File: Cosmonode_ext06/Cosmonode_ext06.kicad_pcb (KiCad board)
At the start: 2 copper layers, 24.1 x 33 mm, 19 parts, among them J1 CONN_01X04, J2 CONN_01X04, J3 CONN_01X08, J4 CONN_01X08, J5 GS3, J6 GS3, Q1 BSS138, Q2 BSS138, SW1 SW_Push, SW2 SW_Push, U1 XC6206P502MR

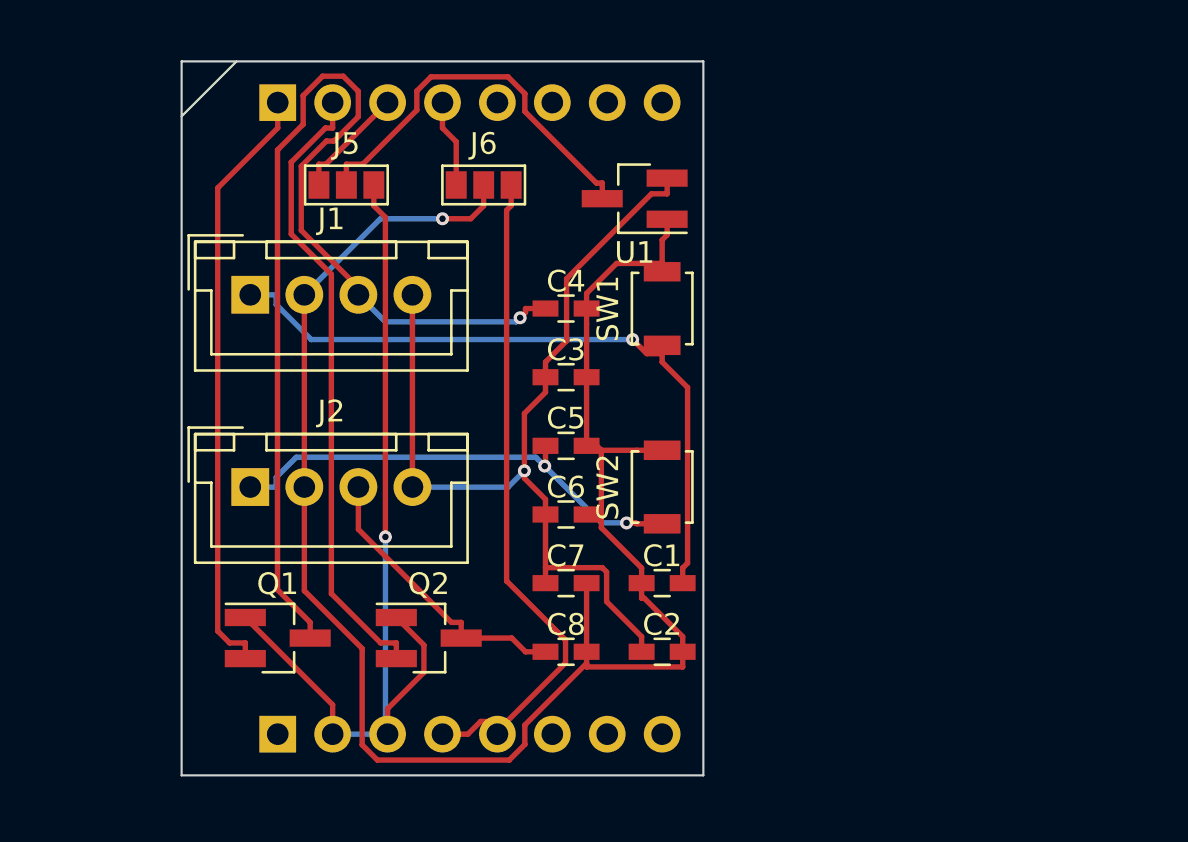
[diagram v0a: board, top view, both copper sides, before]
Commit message: big push2
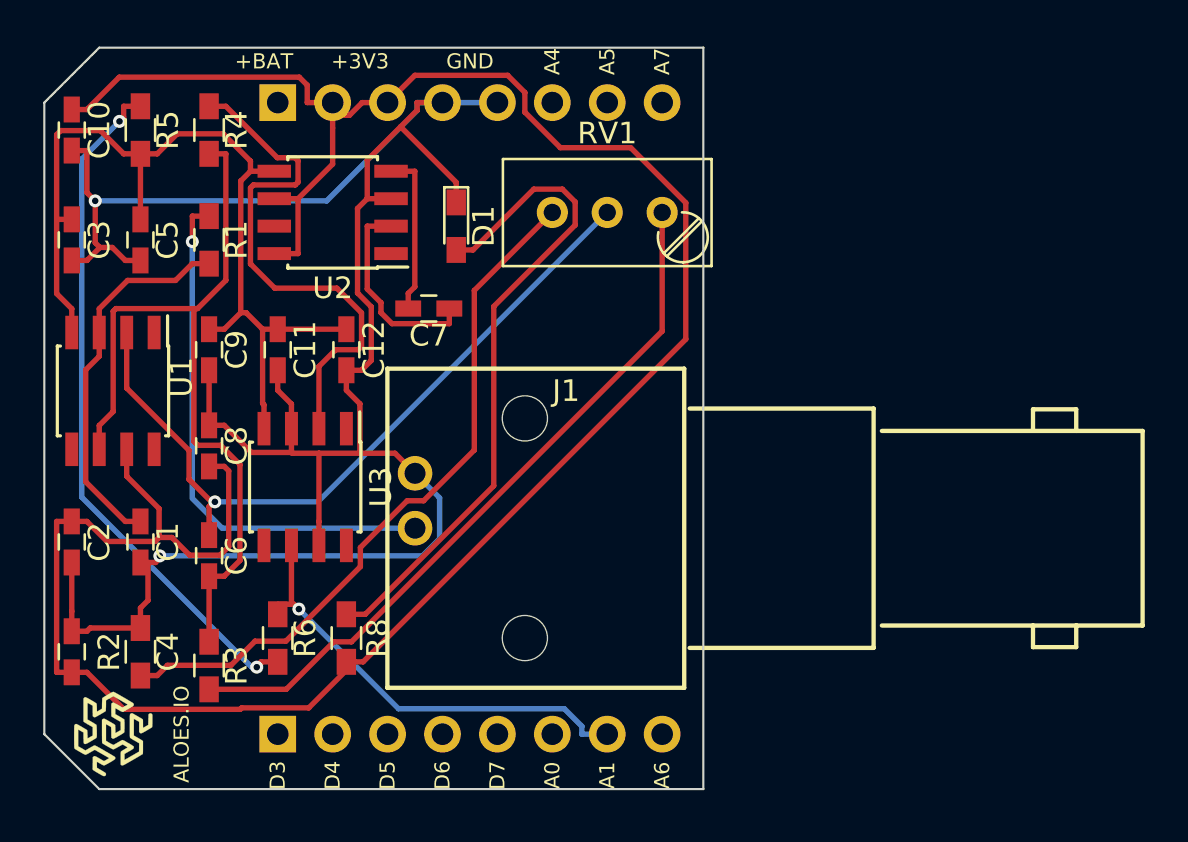
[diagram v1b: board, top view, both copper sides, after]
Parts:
- removed J5: GS3, Connectors:GS3
- removed Q1, Q2: BSS138, TO_SOT_Packages_SMD:SOT-23_Handsoldering
- removed SW1, SW2: SW_Push, Buttons_Switches_SMD:SW_SPST_B3U-1000P
- added C10: 100nF, Capacitors_SMD:C_0603_HandSoldering, F.Cu at (149.2, 92.7)
- added C11: 100nF, Capacitors_SMD:C_0603_HandSoldering, F.Cu at (158.8, 102.9)
- added C12: 100uF, Capacitors_SMD:C_0603_HandSoldering, F.Cu at (161.9, 102.9)
- added C9: 10uF, Capacitors_SMD:C_0603_HandSoldering, F.Cu at (155.6, 102.9)
- added D1: LED, LEDs:LED_0603_HandSoldering, F.Cu at (167.0, 97.2)
- added R1: 4,7M, Resistors_SMD:R_0603_HandSoldering, F.Cu at (155.6, 97.8)
- added R2: 1k, Resistors_SMD:R_0603_HandSoldering, F.Cu at (152.4, 116.8)
- added R3: 2,2k, Resistors_SMD:R_0603_HandSoldering, F.Cu at (155.6, 117.5)
- added R4: 30k, Resistors_SMD:R_0603_HandSoldering, F.Cu at (155.6, 92.7)
- added R5: 75k, Resistors_SMD:R_0603_HandSoldering, F.Cu at (152.4, 92.7)
- added R6: 30k, Resistors_SMD:R_0603_HandSoldering, F.Cu at (158.8, 116.2)
- added R8: 1k, Resistors_SMD:R_0603_HandSoldering, F.Cu at (161.9, 116.2)
- added RV1: 5k, Potentiometers:Potentiometer_Trimmer_Bourns_3296W, F.Cu at (176.5, 96.5)
- added U2: ICL7660AIBAZA, Housings_SOIC:SOIC-8_3.9x4.9mm_Pitch1.27mm, F.Cu at (161.3, 96.5)
- added U3: TL081BCD, Housings_SOIC:SOIC-8_3.9x4.9mm_Pitch1.27mm, F.Cu at (160.0, 109.2)
- C1: value 100nF -> 2,2nF
- C2: value 10uF -> 100nF
- C3, C4, C8: value 100nF -> 10uF
- C6: value 10uF -> 1uF
- C7: value 100nF -> 100uF
- J1: value CONN_01X04 -> 227161-1; footprint Connectors_JST:JST_XH_B04B-XH-A_04x2.50mm_Straight -> BNC_P7003:TE_227161-1
- J2: value CONN_01X04 -> Aloes_Logo; footprint Connectors_JST:JST_XH_B04B-XH-A_04x2.50mm_Straight -> Aloes:Aloes_mini
- J3: value CONN_01X08 -> OSHW_Logo; footprint Pin_Headers:Pin_Header_Straight_1x08_Pitch2.54mm -> Symbols:OSHW-Logo_5.7x6mm_SilkScreen
- J4: footprint Pin_Headers:Pin_Header_Straight_1x08_Pitch2.54mm -> Socket_Strips:Socket_Strip_Straight_1x08_Pitch2.54mm
- J6: value GS3 -> CONN_01X08; footprint Connectors:GS3 -> Socket_Strips:Socket_Strip_Straight_1x08_Pitch2.54mm; moved to B.Cu
- U1: value XC6206P502MR -> CA3140AMZ; footprint TO_SOT_Packages_SMD:SOT-23_Handsoldering -> Housings_SOIC:SOIC-8_3.9x4.9mm_Pitch1.27mm
- moved C4 27.8 mm to (149.2, 116.8), turned to 90 degrees
- moved C2 27.8 mm to (149.2, 111.8), turned to 90 degrees
- moved U1 25.7 mm to (151.1, 104.8), turned to 270 degrees
- moved C1 24.2 mm to (152.4, 111.8), turned to 90 degrees
- moved C3 23.7 mm to (149.2, 97.8), turned to 90 degrees
- moved C5 21.9 mm to (152.4, 97.8), turned to 270 degrees
- moved C8 19.1 mm to (155.6, 107.3), turned to 90 degrees
- moved J1 16.7 mm to (170.2, 111.1), turned to 270 degrees
- moved C6 16.6 mm to (155.6, 112.4), turned to 90 degrees
- moved C7 14.2 mm to (165.7, 101.0), turned to 180 degrees
- moved J2 13.1 mm to (151.1, 120.7), turned to 90 degrees
- moved J6 10.3 mm to (158.8, 91.4), turned to 270 degrees
- moved J3 7.24 mm to (153.0, 95.9)
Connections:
- C1 pad 1: Net-(C1-Pad1) -> GND
- C2 pad 1: +5V -> GND
- C2 pad 2: Net-(C1-Pad1) -> +3V3
- C3 pad 1: +5V -> GND
- C3 pad 2: Net-(C1-Pad1) -> -3V3
- C4 pad 1: /D3_5V -> +3V3
- C4 pad 2: Net-(C1-Pad1) -> GND
- C5 pad 1: Net-(C1-Pad1) -> -3V3
- C5 pad 2: Net-(C5-Pad2) -> GND
- C6 pad 1: +5V -> Net-(C6-Pad1)
- C6 pad 2: Net-(C1-Pad1) -> Net-(C6-Pad2)
- C7 pad 1: +5V -> Net-(C7-Pad1)
- C7 pad 2: Net-(C1-Pad1) -> Net-(C7-Pad2)
- C8 pad 1: /D4_5V -> +3V3
- C8 pad 2: Net-(C1-Pad1) -> GND
- J1 pad 1: Net-(C1-Pad2) -> GND
- J1 pad 2: Net-(C1-Pad1) -> Net-(J1-Pad2)
- J4 pad 1: /BAT+ -> /D3
- J4 pad 2: +3V3 -> /D4
- J4 pad 3: +3V3 -> /D5
- J4 pad 4: GND -> /D6
- J4 pad 5: GND -> /D7
- J4 pad 6: /A4 -> /A0
- J4 pad 7: /A5 -> /A1
- J4 pad 8: /A7 -> /A6
- J6 pad 1: /D6 -> /BAT+
- J6 pad 2: Net-(C1-Pad1) -> +3V3
- J6 pad 3: GND -> +3V3
- U1 pad 1: Net-(C1-Pad1) -> Net-(U1-Pad1)
- U1 pad 2: +5V -> Net-(C6-Pad2)
- U1 pad 3: Net-(J5-Pad2) -> Net-(C1-Pad2)
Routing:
- net Net-(C1-Pad1): track 83.8 -> 0.00 mm, vias 1 -> 0
- net GND: track 31.0 -> 104.2 mm, vias 0 -> 2
- net +3V3: track 41.8 -> 112.3 mm, vias 1 -> 0
- net /D3_5V: track 50.7 -> 0.00 mm, vias 1 -> 0
- net +5V: track 43.9 -> 0.00 mm, vias 1 -> 0
- net -3V3: track 0.00 -> 43.5 mm
- net Net-(C6-Pad1): track 0.00 -> 37.0 mm
- net Net-(C6-Pad2): track 0.00 -> 34.9 mm, vias 0 -> 1
- net Net-(R3-Pad2): track 0.00 -> 33.3 mm
- net Net-(R2-Pad1): track 0.00 -> 32.8 mm
- net Net-(R5-Pad1): track 0.00 -> 32.1 mm, vias 0 -> 2
- net Net-(D1-Pad2): track 0.00 -> 30.9 mm
- net /D4: track 29.1 -> 0.00 mm
- net /D3: track 27.8 -> 0.00 mm
- net Net-(R4-Pad1): track 0.00 -> 24.8 mm
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- added copper zone on B.Cu, net GND
- added copper zone on F.Cu, net GND
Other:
- board size 24.1 x 33 mm -> 30.5 x 34.3 mm
- board text added: "+3V3"
- board text added: "+BAT"
- board text added: "A0"
- board text added: "A1"
- board text added: "A4"
- board text added: "A5"
- board text added: "A6"
- board text added: "A7"
- board text added: "ALOES.IO"
- board text added: "D3"
- board text added: "D4"
- board text added: "D5"
- board text added: "D6"
- board text added: "D7"
- board text added: "Extension #7 pH sensor driver BNC probe"
- board text added: "GND"
